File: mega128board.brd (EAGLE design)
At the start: 83.8 x 100.3 mm, 6 parts, among them IC1 MEGA128-A

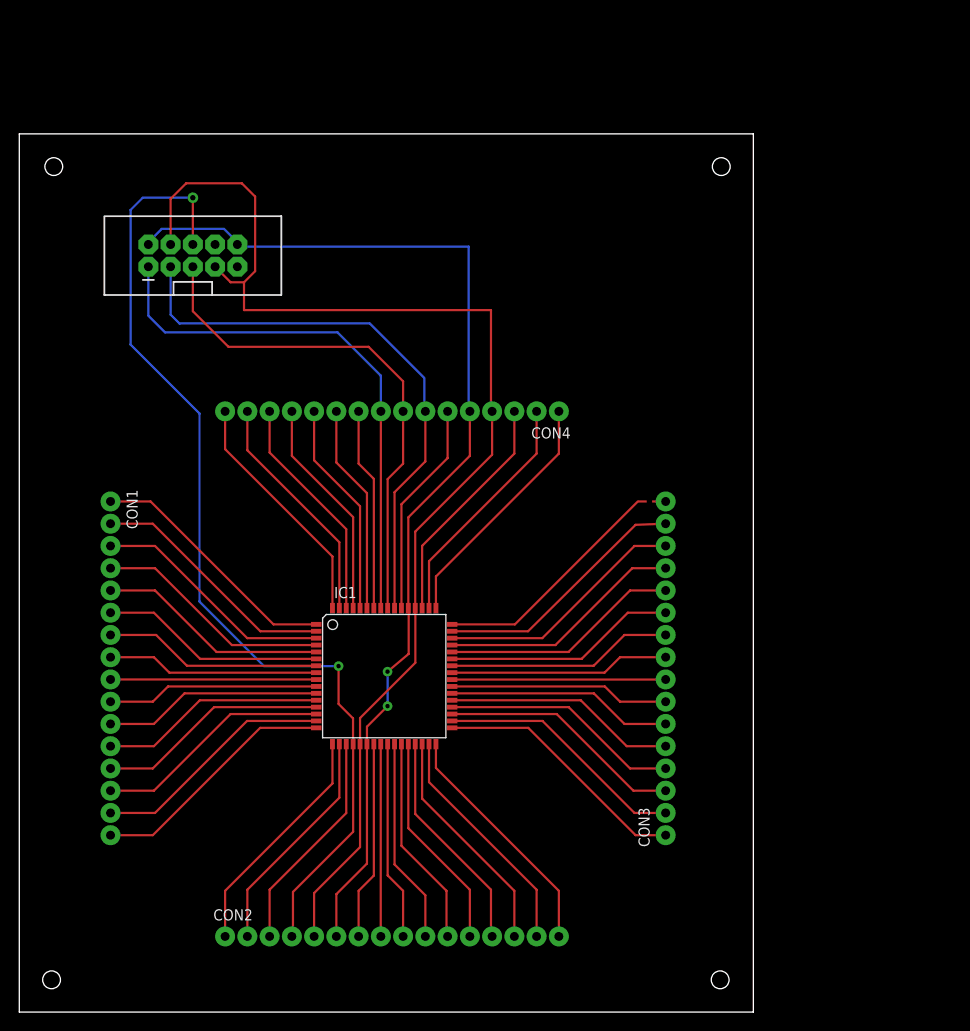
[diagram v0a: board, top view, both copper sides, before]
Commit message: ~
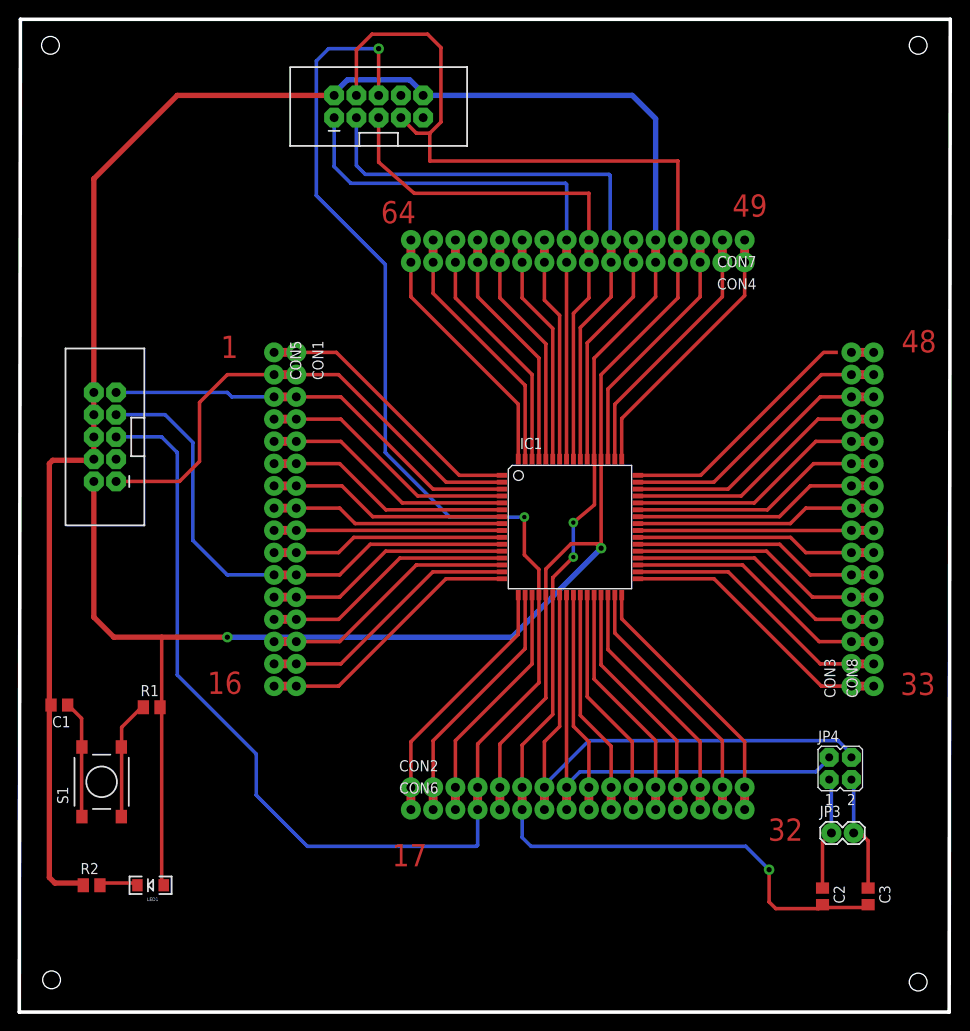
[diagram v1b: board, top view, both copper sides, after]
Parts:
- added C1, C2, C3: (no value), rcl:C0805
- added CON5, CON6, CON7, CON8: (no value), SparkFun-Connectors:1X16_NO_SILK
- added ICSP: (no value), SparkFun-Connectors:2X5-SHROUDED
- added JP3: M02PTH, SparkFun-Connectors:1X02
- added JP4: (no value), jumper:JP2Q
- added LED1: (no value), SparkFun-LED:LED-1206
- added R1, R2: (no value), rcl:M0805
- added S1: DTSM-6, switch-tact:DTSM-6
- moved CON1 27.2 mm to (31.6, 75.3)
- moved CON4 27.2 mm to (82.8, 85.6)
- moved IC1 27.2 mm to (62.9, 55.4)
- moved CON2 27.2 mm to (44.7, 25.7)
- moved JTAG 27.2 mm to (41.0, 103.4)
- moved CON3 27.2 mm to (95.0, 37.2)
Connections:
- new net N$1: C1.1, S1.1, S1.2
- new net N$2: R1.1, S1.3, S1.4
- new net N$3: LED1.C, R2.2
- new net N$5: C3.1, JP3.2, JP4.3
- new net N$6: C2.1, JP3.1, JP4.1
- net +5V: now also CON6.5, CON7.4, ICSP.2, LED1.A, R1.2
- net AGND: now also CON7.15
- net ALE: now also CON8.11
- net AREF: now also CON7.14
- net AVCC: now also CON7.16
- net GND: now also C1.2, C2.2, C3.2, CON6.6, CON7.5, ICSP.10, ICSP.4, ICSP.6, ICSP.8, R2.1
- net PA0: now also CON7.3
- net PA1: now also CON7.2
- net PA2: now also CON7.1
- net PA3: now also CON8.16
- net PA4: now also CON8.15
- net PA5: now also CON8.14
- net PA6: now also CON8.13
- net PA7: now also CON8.12
- net PB0: now also CON5.10
- net PB1: now also CON5.11, ICSP.7
- net PB2: now also CON5.12
- net PB3: now also CON5.13
- net PB4: now also CON5.14
- net PB5: now also CON5.15
- net PB6: now also CON5.16
- net PB7: now also CON6.1
- net PC0: now also CON8.3
- net PC1: now also CON8.4
- net PC2: now also CON8.5
- net PC3: now also CON8.6
- net PC4: now also CON8.7
- net PC5: now also CON8.8
- net PC6: now also CON8.9
- net PC7: now also CON8.10
- net PD0: now also CON6.9
- net PD1: now also CON6.10
- net PD2: now also CON6.11
- net PD3: now also CON6.12
- net PD4: now also CON6.13
- net PD5: now also CON6.14
- net PD6: now also CON6.15
- net PD7: now also CON6.16
- net PE0: now also CON5.2, ICSP.1
- net PE1: now also CON5.3, ICSP.9
- net PE2: now also CON5.4
- net PE3: now also CON5.5
- net PE4: now also CON5.6
- net PE5: now also CON5.7
- net PE6: now also CON5.8
- net PE7: now also CON5.9
- net PEN: now also CON5.1
- net PF0: now also CON7.13
- net PF1: now also CON7.12
- net PF2: now also CON7.11
- net PF3: now also CON7.10
- net RD: now also CON8.2
- net RESET: now also CON6.4, ICSP.5
- net TCK: now also CON7.9
- net TDI: now also CON7.6
- net TDO: now also CON7.7
- net TMS: now also CON7.8
- net TOSC1: now also CON6.3
- net TOSC2: now also CON6.2
- net WR: now also CON8.1
- net XTAL1: now also CON6.8, JP4.2
- net XTAL2: now also CON6.7, JP4.4
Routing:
- net GND: track 123.9 -> 298.1 mm, vias 2 -> 3
- net +5V: track 142.0 -> 254.2 mm, vias 0 -> 2
- net RESET: track 114.5 -> 202.4 mm
- net XTAL2: track 22.7 -> 63.6 mm
- net PB1: track 24.9 -> 62.2 mm
- net XTAL1: track 22.0 -> 56.1 mm
- net PE0: track 28.6 -> 58.1 mm
- net PE1: track 27.8 -> 48.6 mm
- net N$5: track 0.00 -> 13.8 mm
- net N$2: track 0.00 -> 13.6 mm
- net N$1: track 0.00 -> 13.5 mm
- net N$6: track 0.00 -> 13.1 mm
- net N$3: track 0.00 -> 4.45 mm
- net TDO: track 65.3 -> 69.0 mm
- net TCK: track 61.5 -> 64.3 mm
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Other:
- board size 83.8 x 100.3 mm -> 106.3 x 113.3 mm
- board text added: "1"
- board text added: "16"
- board text added: "17"
- board text added: "32"
- board text added: "33"
- board text added: "48"
- board text added: "49"
- board text added: "64"
